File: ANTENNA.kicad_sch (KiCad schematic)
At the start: 16 parts, among them J7 SMA-J-P-X-RA-TH1, Q1 MMBT3904LT1G, Q9 PMOS, U15 TPS22946YZPR, U9 MCP6001-OT

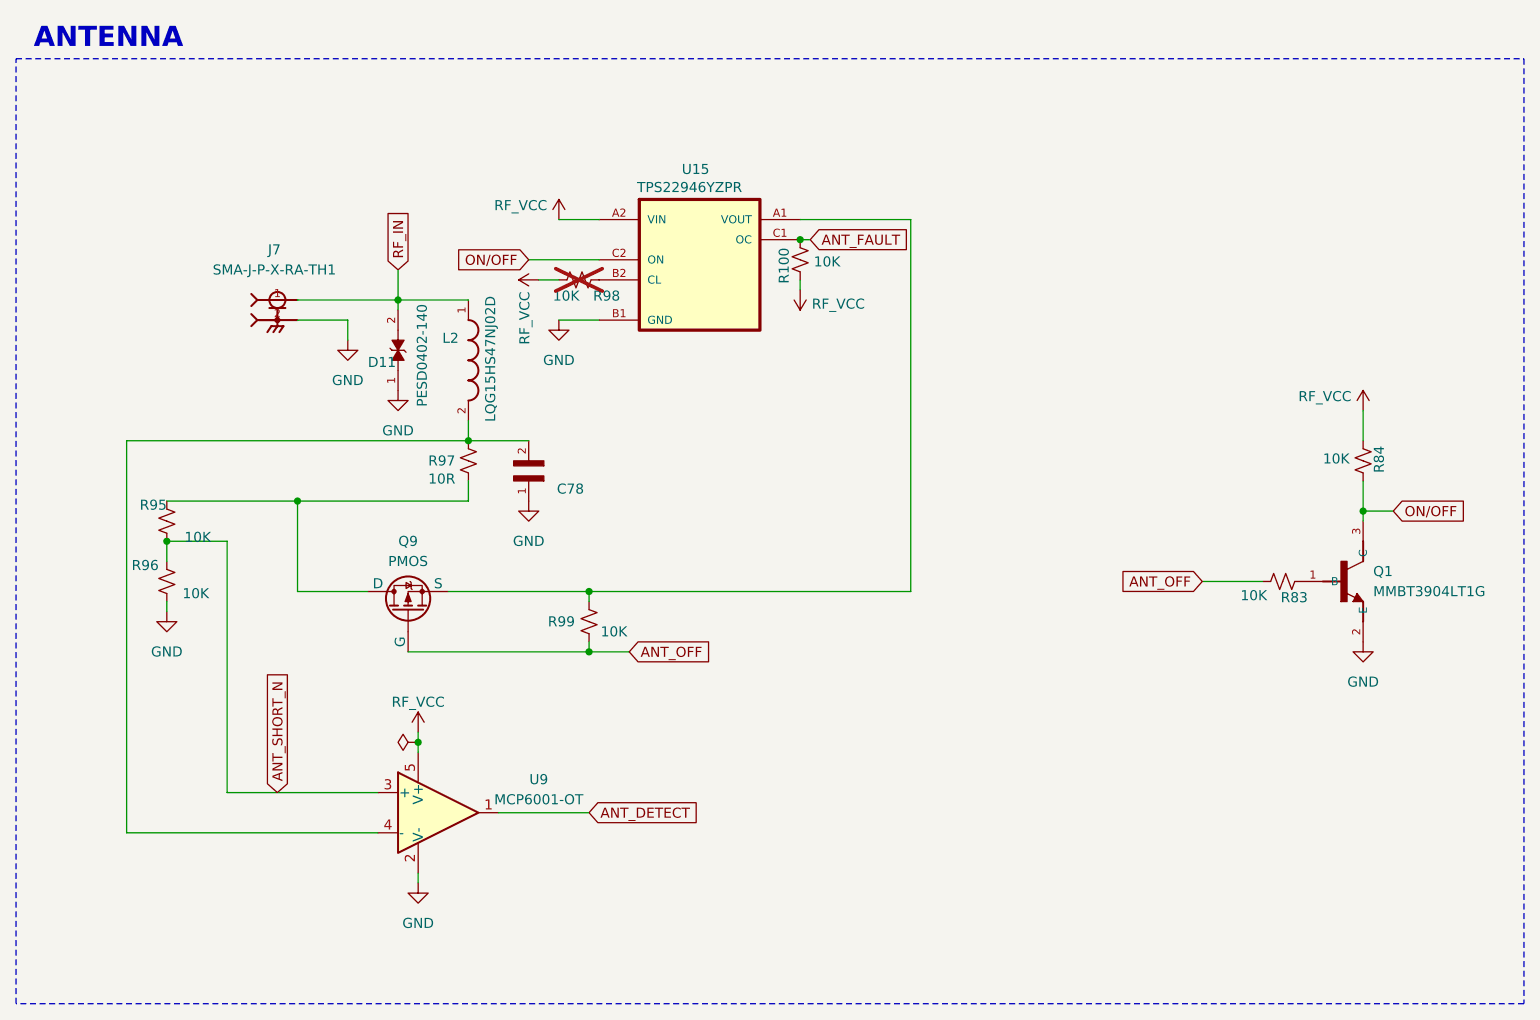
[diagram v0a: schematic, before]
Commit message: 18.09.2026
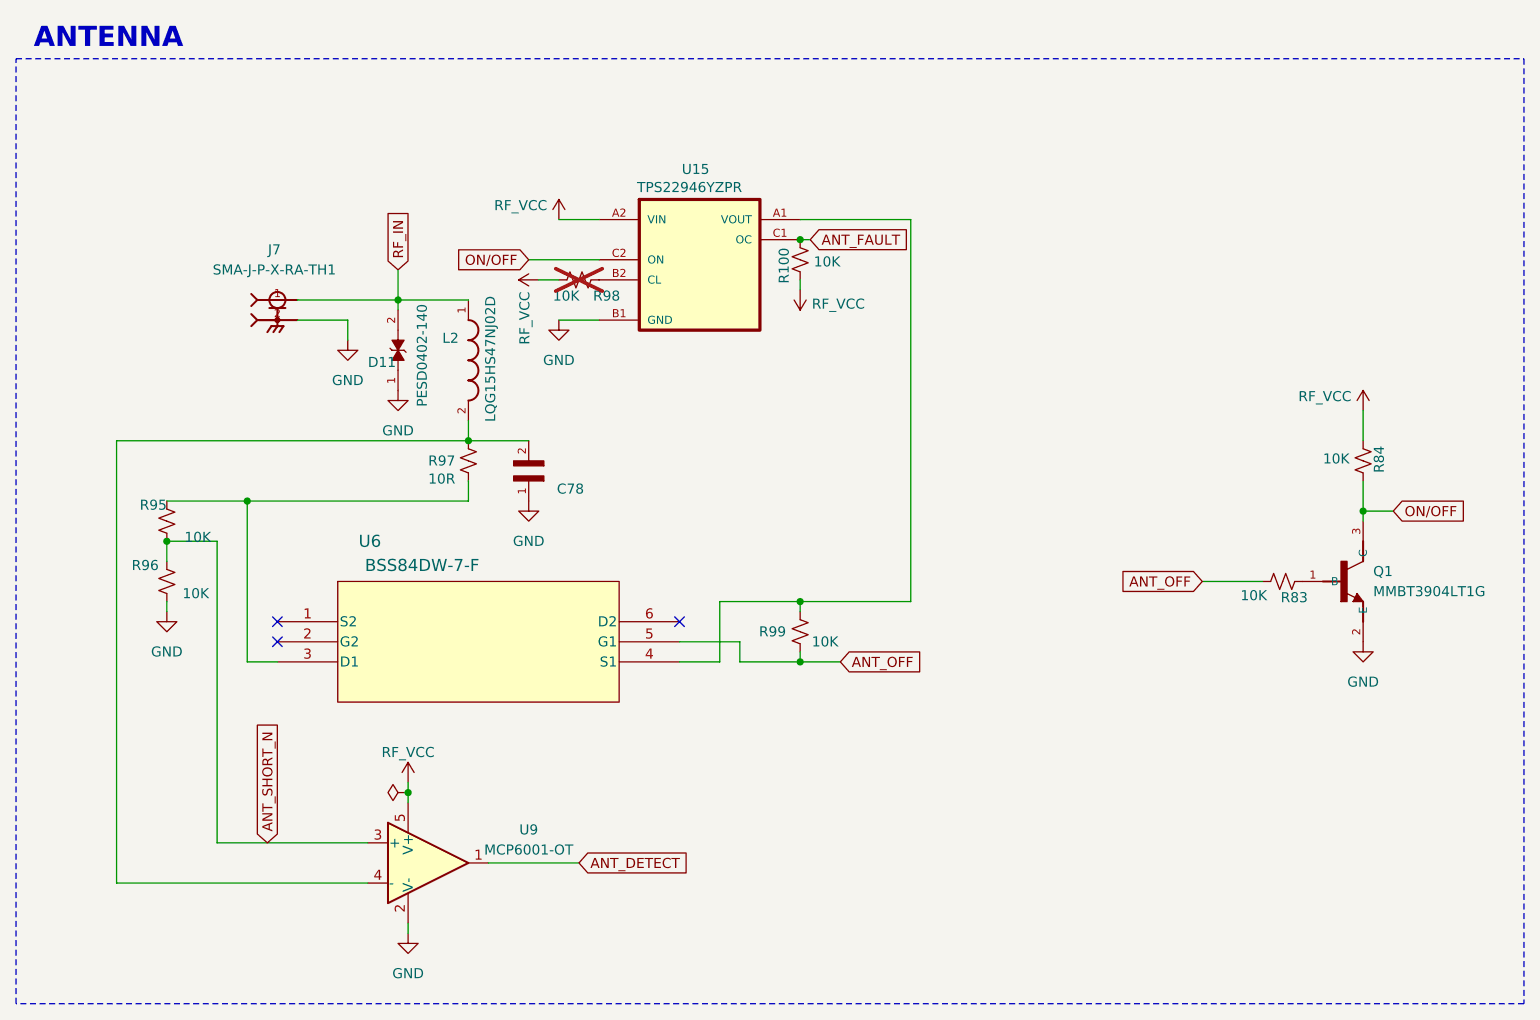
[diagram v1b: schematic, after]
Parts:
- removed Q9: PMOS, symbol Simulation_SPICE:PMOS
- added U6: BSS84DW-7-F, SOT-363_DIO, symbol 2026-09-17_17-18-21:BSS84DW-7-F
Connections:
- net ANT_OFF: now also U6.5 (G1)
- net at R95.2, R97.2: now also U6.3 (D1)
- net at R99.2, U15.A1 (VOUT): now also U6.4 (S1)
- no-connect marks 0 -> 3
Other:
- moved on the sheet: R99, U9
